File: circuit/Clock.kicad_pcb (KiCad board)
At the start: 2 copper layers, 122.4 x 32 mm, 26 parts, among them SW1 SW_Push, SW2 SW_Push, SW3 SW_Push, SW4 SW_Push, U2 Max98357

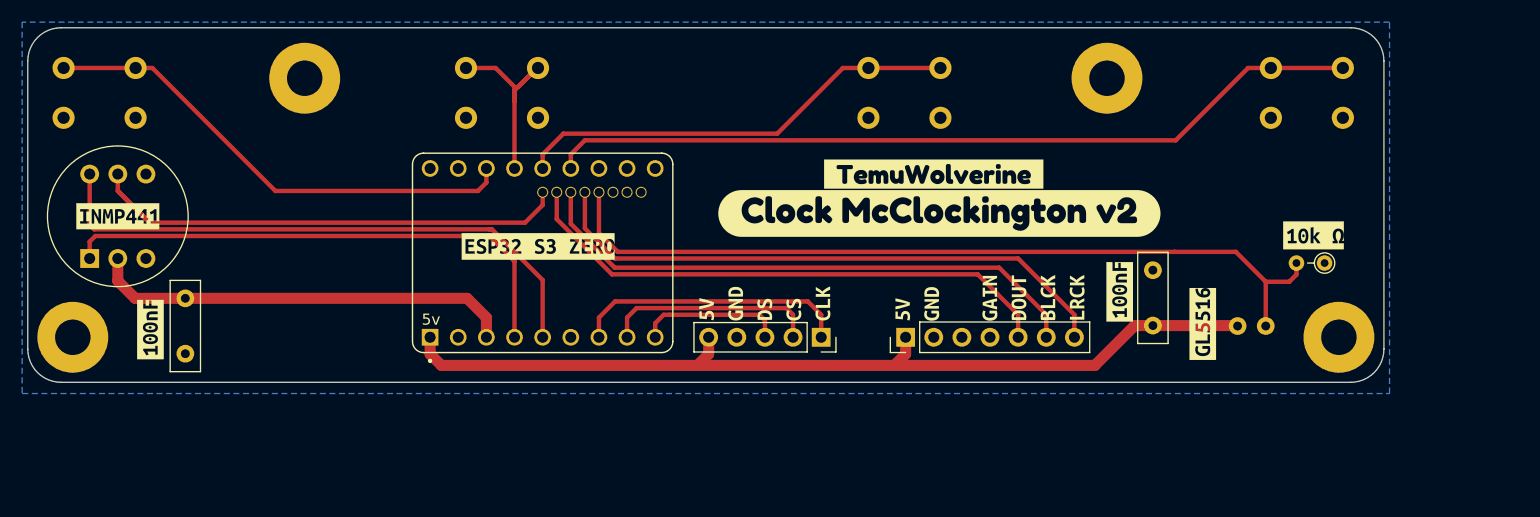
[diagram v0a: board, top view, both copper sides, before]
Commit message: design sent to mfg
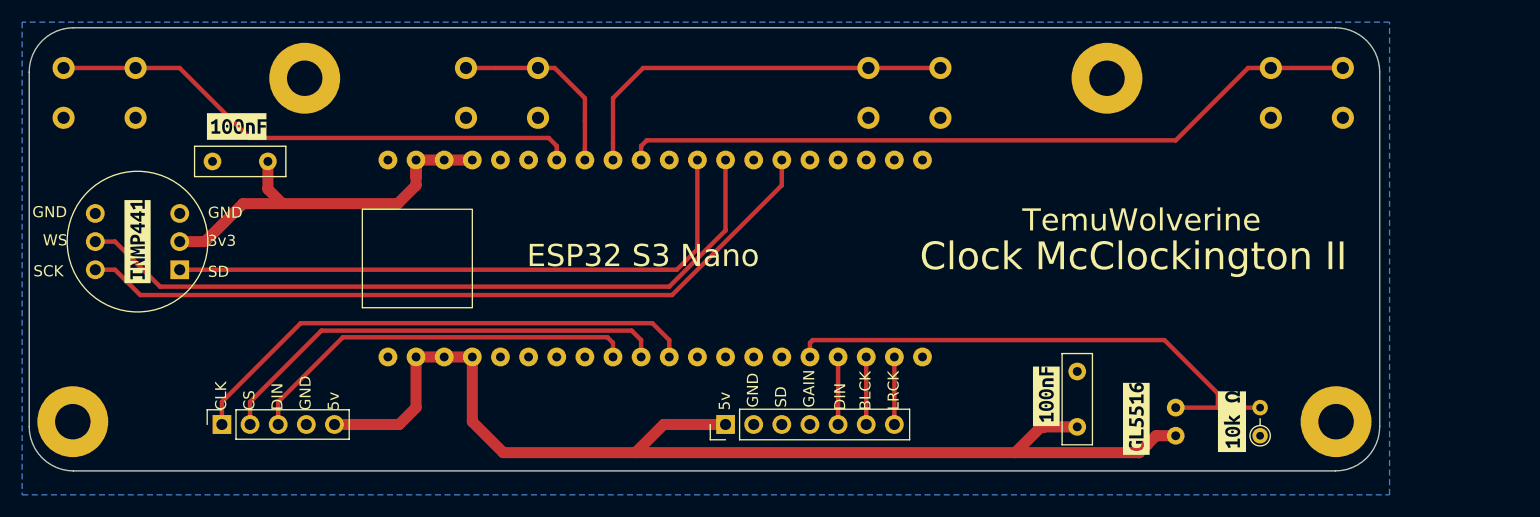
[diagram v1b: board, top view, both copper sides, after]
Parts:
- removed ESP32_S1: ~, PaulsCoolKicadLibrary:MODULE_ESP32-S3-ZERO
- removed kibuzzard-69B4FF18: G***, kibuzzard-69B4FF18
- removed kibuzzard-69B4FF3C: G***, kibuzzard-69B4FF3C
- removed kibuzzard-69B50323: G***, kibuzzard-69B50323
- removed kibuzzard-69B50368: G***, kibuzzard-69B50368
- removed kibuzzard-69B74ACD: G***, kibuzzard-69B74ACD
- added U1: ESP32_S3_NANO, Paul:ESP32_S3_NANO, F.Cu at (171.4, 108.4)
- M1: footprint PaulsCoolKicadLibrary:INMP441 -> Paul:INMP441
- moved Display1 54.7 mm to (132.3, 123.4), turned to 90 degrees
- moved kibuzzard-69B74B24 19.9 mm to (133.6, 96.5), turned to 0 degrees
- moved kibuzzard-69B74B07 18.4 mm to (223.4, 123.1), turned to 90 degrees
- moved U2 18.1 mm to (177.7, 123.4)
- moved 10k1 16.6 mm to (226.0, 124.4), turned to 90 degrees
- moved C1 14.4 mm to (136.4, 99.6), turned to 180 degrees
- moved kibuzzard-69B74B24 11.5 mm to (206.7, 120.8)
- moved C2 11.4 mm to (209.5, 123.6)
- moved R1 11.0 mm to (218.4, 121.8), turned to -90 degrees
- moved kibuzzard-69B74AF7 10.5 mm to (214.8, 122.9)
- moved M1 8.19 mm to (128.4, 109.4), turned to 180 degrees
- moved H2 7.62 mm to (232.8, 123.1)
- moved H3 7.62 mm to (118.8, 123.1)
- moved kibuzzard-69B74AE8 2.90 mm to (124.6, 106.9), turned to 90 degrees
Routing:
- net LRCK: track 52.7 -> 6.10 mm
- net BLCK: track 51.2 -> 6.10 mm
- net SPK_DOUT: track 49.7 -> 6.10 mm
- net PhotoresistorSignal: track 73.8 -> 49.1 mm
- net DisplaySignal: track 13.2 -> 36.2 mm
- net Clock: track 25.0 -> 47.5 mm
- net CS: track 19.4 -> 41.9 mm
- net +5V: track 82.3 -> 104.5 mm
- net WS: track 46.5 -> 67.0 mm
- net SCK: track 52.7 -> 69.3 mm
- net MIC_DIN: track 47.9 -> 55.5 mm
- net btnFour: track 74.1 -> 67.5 mm
- net btnOne: track 44.4 -> 48.8 mm
- net btnThree: track 40.3 -> 36.2 mm
- net +3V3: track 38.5 -> 35.9 mm
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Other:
- board size 122.4 x 32 mm -> 121.9 x 40 mm
- board text added: "3v3"
- board text added: "5v"
- board text added: "BLCK"
- board text added: "CLK"
- board text added: "CS"
- board text added: "Clock McClockington II"
- board text added: "DIN"
- board text added: "ESP32 S3 Nano"
- board text added: "GAIN"
- board text added: "GND"
- board text added: "LRCK"
- board text added: "SCK"
- board text added: "SD"
- board text added: "TemuWolverine"
- board text added: "WS"
